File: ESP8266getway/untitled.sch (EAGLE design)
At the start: 18 parts, among them IC1 LM1117MP-3.3

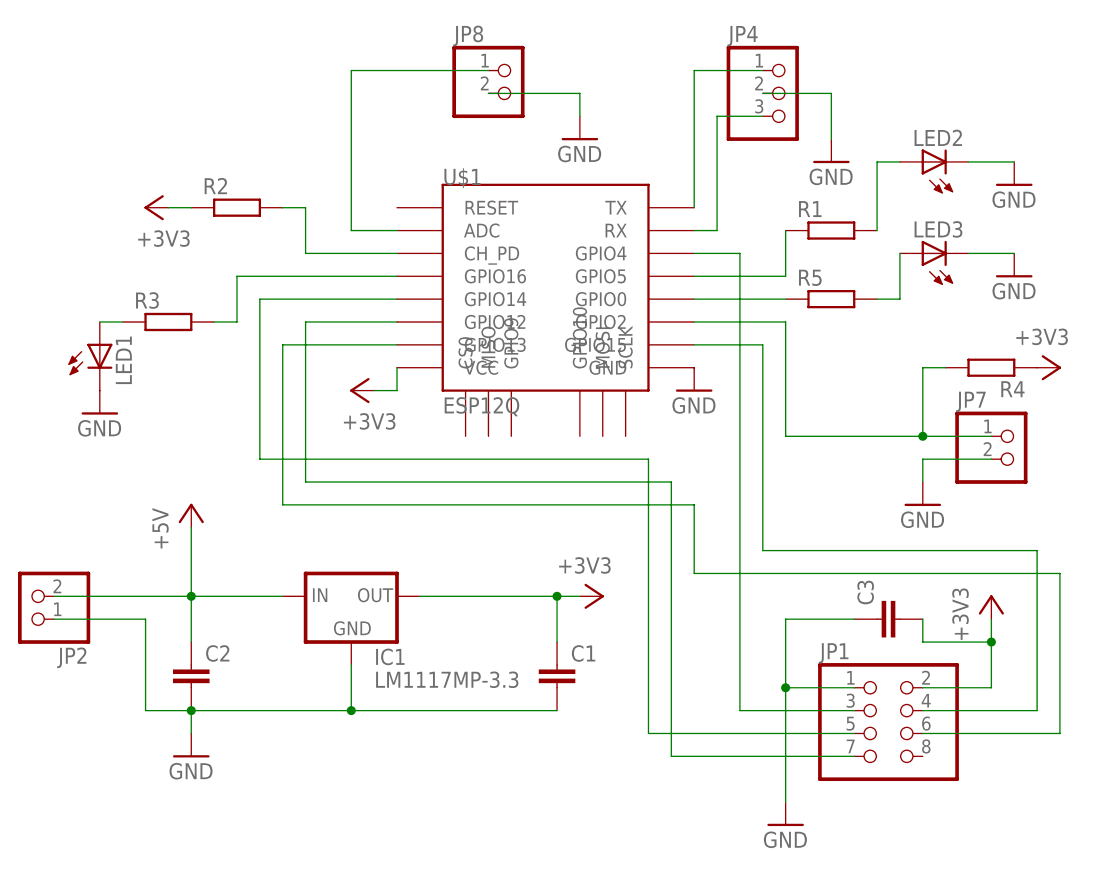
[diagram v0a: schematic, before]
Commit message: 2092017
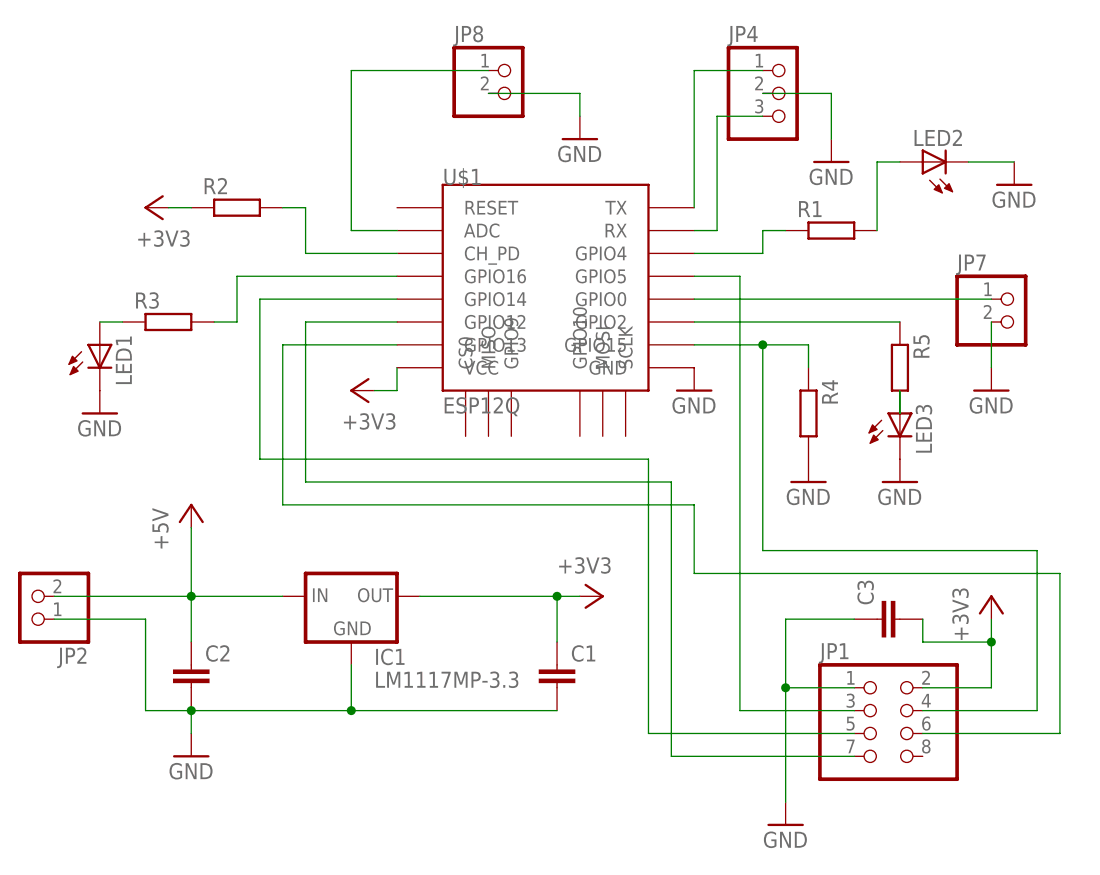
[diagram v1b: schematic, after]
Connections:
- removed net N$14: R1.1, U$1.GPIO5
- new net N$25: R1.1, U$1.GPIO4
- net +3V3: no longer R4.1
- net GND: now also R4.2
- net N$1: now also U$1.GPIO5; no longer U$1.GPIO4
- net N$11: now also R5.1; no longer JP7.1, R4.2
- net N$2: now also R4.1
- net N$3: now also JP7.1; no longer R5.1
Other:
- moved on the sheet: JP7, LED3, R4, R5
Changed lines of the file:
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@@
 <part name="JP7" library="pinhead" deviceset="PINHD-1X2" device=""/>
 <part name="R4" library="rcl" deviceset="R-EU_" device="M0805"/>
-<part name="+3V5" library="supply1" deviceset="+3V3" device=""/>
 <part name="GND5" library="supply1" deviceset="GND" device=""/>
 <part name="R5" library="rcl" deviceset="R-EU_" device="R0805"/>
@@
 <part name="LED3" library="led" deviceset="LED" device="SFH482"/>
 <part name="C3" library="rcl" deviceset="C-EU" device="C3216"/>
+<part name="GND10" library="supply1" deviceset="GND" device=""/>
 </parts>
 <sheets>
@@
 <instance part="R3" gate="G$1" x="-50.8" y="81.28"/>
 <instance part="GND4" gate="1" x="-58.42" y="71.12"/>
-<instance part="JP7" gate="G$1" x="43.18" y="66.04"/>
-<instance part="R4" gate="G$1" x="40.64" y="76.2" rot="R180"/>
-<instance part="+3V5" gate="G$1" x="48.26" y="76.2" rot="R270"/>
-<instance part="GND5" gate="1" x="33.02" y="60.96"/>
-<instance part="R5" gate="G$1" x="22.86" y="83.82"/>
-<instance part="GND6" gate="1" x="43.18" y="86.36"/>
+<instance part="JP7" gate="G$1" x="43.18" y="81.28"/>
+<instance part="R4" gate="G$1" x="20.32" y="71.12" rot="R270"/>
+<instance part="GND5" gate="1" x="40.64" y="73.66"/>
+<instance part="R5" gate="G$1" x="30.48" y="76.2" rot="R270"/>
+<instance part="GND6" gate="1" x="30.48" y="63.5"/>
 <instance part="GND7" gate="1" x="43.18" y="96.52"/>
 <instance part="R1" gate="G$1" x="22.86" y="91.44"/>
@@
 <instance part="LED1" gate="G$1" x="-58.42" y="78.74"/>
 <instance part="LED2" gate="G$1" x="33.02" y="99.06" rot="R90"/>
-<instance part="LED3" gate="G$1" x="33.02" y="88.9" rot="R90"/>
+<instance part="LED3" gate="G$1" x="30.48" y="71.12"/>
 <instance part="C3" gate="G$1" x="27.94" y="48.26" rot="R90"/>
+<instance part="GND10" gate="1" x="20.32" y="63.5"/>
 </instances>
 <busses>
@@
 <segment>
 <pinref part="JP7" gate="G$1" pin="2"/>
-<wire x1="40.64" y1="66.04" x2="33.02" y2="66.04" width="0.1524" layer="91"/>
+<wire x1="40.64" y1="81.28" x2="40.64" y2="76.2" width="0.1524" layer="91"/>
 <pinref part="GND5" gate="1" pin="GND"/>
-<wire x1="33.02" y1="66.04" x2="33.02" y2="63.5" width="0.1524" layer="91"/>
 </segment>
 <segment>
@@
 <pinref part="GND6" gate="1" pin="GND"/>
 <pinref part="LED3" gate="G$1" pin="C"/>
-<wire x1="43.18" y1="88.9" x2="38.1" y2="88.9" width="0.1524" layer="91"/>
 </segment>
 <segment>
@@
 <wire x1="15.24" y1="106.68" x2="22.86" y2="106.68" width="0.1524" layer="91"/>
 <wire x1="22.86" y1="106.68" x2="22.86" y2="101.6" width="0.1524" layer="91"/>
+</segment>
+<segment>
+<pinref part="GND10" gate="1" pin="GND"/>
+<pinref part="R4" gate="G$1" pin="2"/>
 </segment>
 </net>
@@
 </segment>
 <segment>
-<pinref part="R4" gate="G$1" pin="1"/>
-<pinref part="+3V5" gate="G$1" pin="+3V3"/>
-</segment>
-<segment>
 <pinref part="R2" gate="G$1" pin="1"/>
 <pinref part="+3V4" gate="G$1" pin="+3V3"/>
@@
 <pinref part="JP1" gate="A" pin="3"/>
 <wire x1="25.4" y1="38.1" x2="12.7" y2="38.1" width="0.1524" layer="91"/>
-<wire x1="12.7" y1="38.1" x2="12.7" y2="88.9" width="0.1524" layer="91"/>
-<pinref part="U$1" gate="G$1" pin="GPIO4"/>
-<wire x1="12.7" y1="88.9" x2="7.62" y2="88.9" width="0.1524" layer="91"/>
+<pinref part="U$1" gate="G$1" pin="GPIO5"/>
+<wire x1="7.62" y1="86.36" x2="12.7" y2="86.36" width="0.1524" layer="91"/>
+<wire x1="12.7" y1="86.36" x2="12.7" y2="38.1" width="0.1524" layer="91"/>
 </segment>
 </net>
@@
 <pinref part="U$1" gate="G$1" pin="GPIO15"/>
 <wire x1="15.24" y1="78.74" x2="7.62" y2="78.74" width="0.1524" layer="91"/>
+<pinref part="R4" gate="G$1" pin="1"/>
+<wire x1="20.32" y1="76.2" x2="20.32" y2="78.74" width="0.1524" layer="91"/>
+<wire x1="20.32" y1="78.74" x2="15.24" y2="78.74" width="0.1524" layer="91"/>
+<junction x="15.24" y="78.74"/>
 </segment>
 </net>
@@
 </segment>
 </net>
-<net name="N$11" class="0">
-<segment>
-<pinref part="JP7" gate="G$1" pin="1"/>
-<pinref part="U$1" gate="G$1" pin="GPIO2"/>
-<wire x1="7.62" y1="81.28" x2="17.78" y2="81.28" width="0.1524" layer="91"/>
-<wire x1="17.78" y1="81.28" x2="17.78" y2="68.58" width="0.1524" layer="91"/>
-<wire x1="17.78" y1="68.58" x2="33.02" y2="68.58" width="0.1524" layer="91"/>
-<pinref part="R4" gate="G$1" pin="2"/>
-<wire x1="33.02" y1="68.58" x2="40.64" y2="68.58" width="0.1524" layer="91"/>
-<wire x1="35.56" y1="76.2" x2="33.02" y2="76.2" width="0.1524" layer="91"/>
-<wire x1="33.02" y1="76.2" x2="33.02" y2="68.58" width="0.1524" layer="91"/>
-<junction x="33.02" y="68.58"/>
-</segment>
-</net>
-<net name="N$3" class="0">
-<segment>
-<pinref part="U$1" gate="G$1" pin="GPIO0"/>
-<pinref part="R5" gate="G$1" pin="1"/>
-<wire x1="7.62" y1="83.82" x2="17.78" y2="83.82" width="0.1524" layer="91"/>
-</segment>
-</net>
 <net name="N$12" class="0">
 <segment>
 <pinref part="R5" gate="G$1" pin="2"/>
-<wire x1="27.94" y1="83.82" x2="30.48" y2="83.82" width="0.1524" layer="91"/>
 <pinref part="LED3" gate="G$1" pin="A"/>
-<wire x1="30.48" y1="83.82" x2="30.48" y2="88.9" width="0.1524" layer="91"/>
-</segment>
-</net>
-<net name="N$14" class="0">
-<segment>
-<pinref part="U$1" gate="G$1" pin="GPIO5"/>
-<pinref part="R1" gate="G$1" pin="1"/>
-<wire x1="7.62" y1="86.36" x2="17.78" y2="86.36" width="0.1524" layer="91"/>
-<wire x1="17.78" y1="86.36" x2="17.78" y2="91.44" width="0.1524" layer="91"/>
+<wire x1="30.48" y1="71.12" x2="30.48" y2="73.66" width="0.1524" layer="91"/>
 </segment>
 </net>
@@
 </segment>
 </net>
+<net name="N$3" class="0">
+<segment>
+<pinref part="JP7" gate="G$1" pin="1"/>
+<pinref part="U$1" gate="G$1" pin="GPIO0"/>
+<wire x1="40.64" y1="83.82" x2="7.62" y2="83.82" width="0.1524" layer="91"/>
+</segment>
+</net>
+<net name="N$11" class="0">
+<segment>
+<pinref part="R5" gate="G$1" pin="1"/>
+<pinref part="U$1" gate="G$1" pin="GPIO2"/>
+<wire x1="30.48" y1="81.28" x2="7.62" y2="81.28" width="0.1524" layer="91"/>
+</segment>
+</net>
+<net name="N$25" class="0">
+<segment>
+<pinref part="U$1" gate="G$1" pin="GPIO4"/>
+<wire x1="15.24" y1="88.9" x2="7.62" y2="88.9" width="0.1524" layer="91"/>
+<pinref part="R1" gate="G$1" pin="1"/>
+<wire x1="17.78" y1="91.44" x2="15.24" y2="91.44" width="0.1524" layer="91"/>
+<wire x1="15.24" y1="91.44" x2="15.24" y2="88.9" width="0.1524" layer="91"/>
+</segment>
+</net>
